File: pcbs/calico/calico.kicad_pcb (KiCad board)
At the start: 2 copper layers, 135 x 102.1 mm, 61 parts, among them J1 MJ-4PP-9-kbd-corne-light-resc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, SW1 SW_Push, SW10 SW_Push, SW11 SW_Push, SW12 SW_Push, SW13 SW_Push, SW14 SW_Push, SW15 SW_Push, SW16 SW_Push, SW17 SW_Push, SW18 SW_Push, SW19 SW_Push, SW2 SW_Push, SW20 SW_Push, SW21 SW_Push, SW22 SW_Push, SW23 SW_Push, SW24 SW_Push, SW25 SW_Push, SW26 SW_Push, SW27 SW_Push, SW3 SW_Push, SW4 SW_Push, SW5 SW_Push, SW6 SW_Push, SW7 SW_Push, SW8 SW_Push, SW9 SW_Push

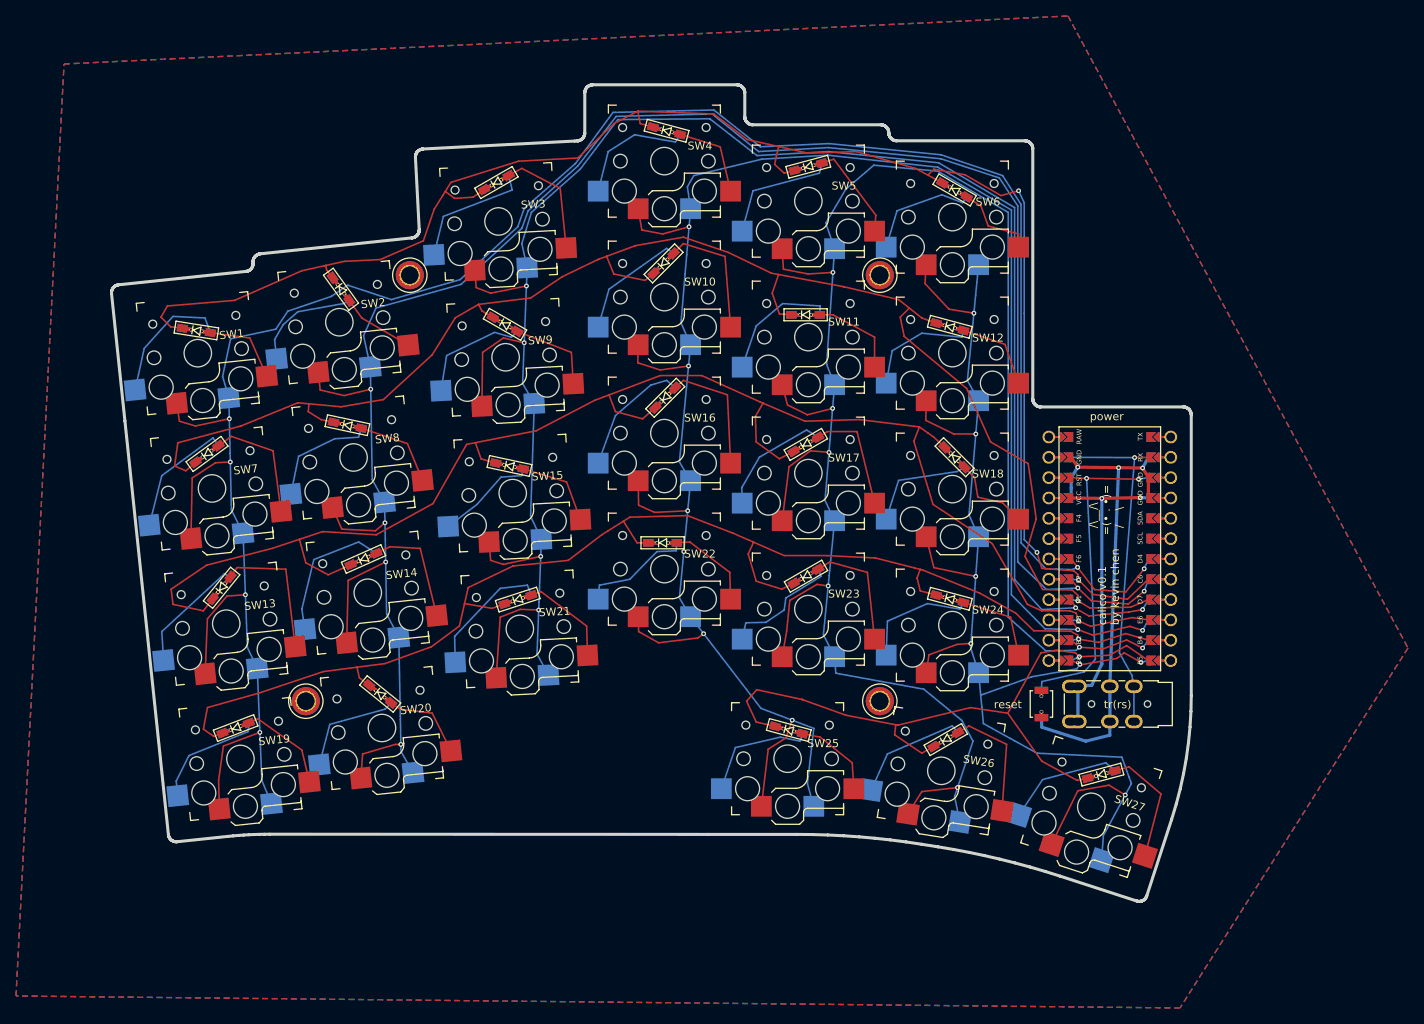
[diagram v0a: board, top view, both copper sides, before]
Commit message: v0.2 initial
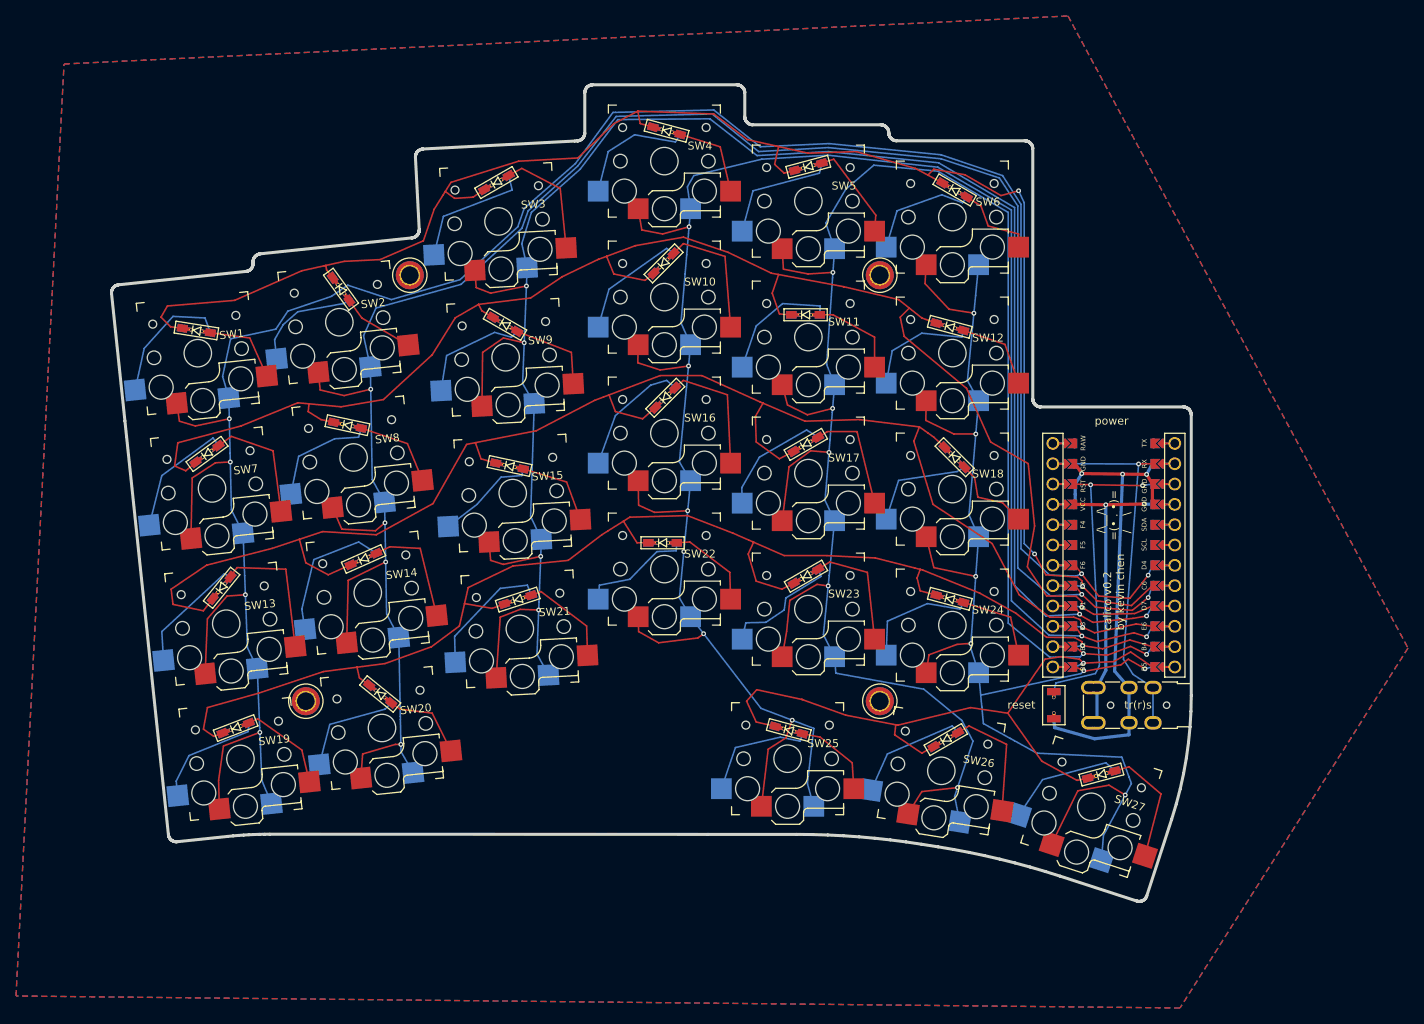
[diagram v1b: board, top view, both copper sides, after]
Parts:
- J1: footprint calico:TRRS-3pin -> calico:TRRS-3pin_modified
- RSW1: footprint calico:Reset -> calico:Reset_modified
- U1: footprint calico:ProMicro_jumpers_modified -> calico:ProMicro_jumpers
- moved J1 2.39 mm to (158.6, 95.0)
- moved RSW1 1.56 mm to (143.0, 95.0)
- moved U1 0.94 mm to (150.5, 76.2)
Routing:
- net +5V: track 39.4 -> 37.2 mm
- net /RESET: track 41.0 -> 39.6 mm
- net /COL1: track 238.3 -> 239.4 mm
- net /COL4: track 258.1 -> 259.2 mm
- net /COL2: track 248.7 -> 249.9 mm
- net /COL5: track 286.3 -> 287.4 mm
- net /COL3: track 237.6 -> 238.7 mm
- net /ROW4: track 205.4 -> 206.4 mm
- net /ROW3: track 191.4 -> 192.2 mm
- net /ROW2: track 192.0 -> 192.7 mm
- net /ROW1: track 164.0 -> 164.7 mm
- net /RX: track 43.2 -> 43.8 mm
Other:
- board text added: "calico v0.2 by kevin chen"
- board text removed: "calico v0.1 by kevin chen"
- board text removed: "tr(rs)"

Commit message: v0.2 updated
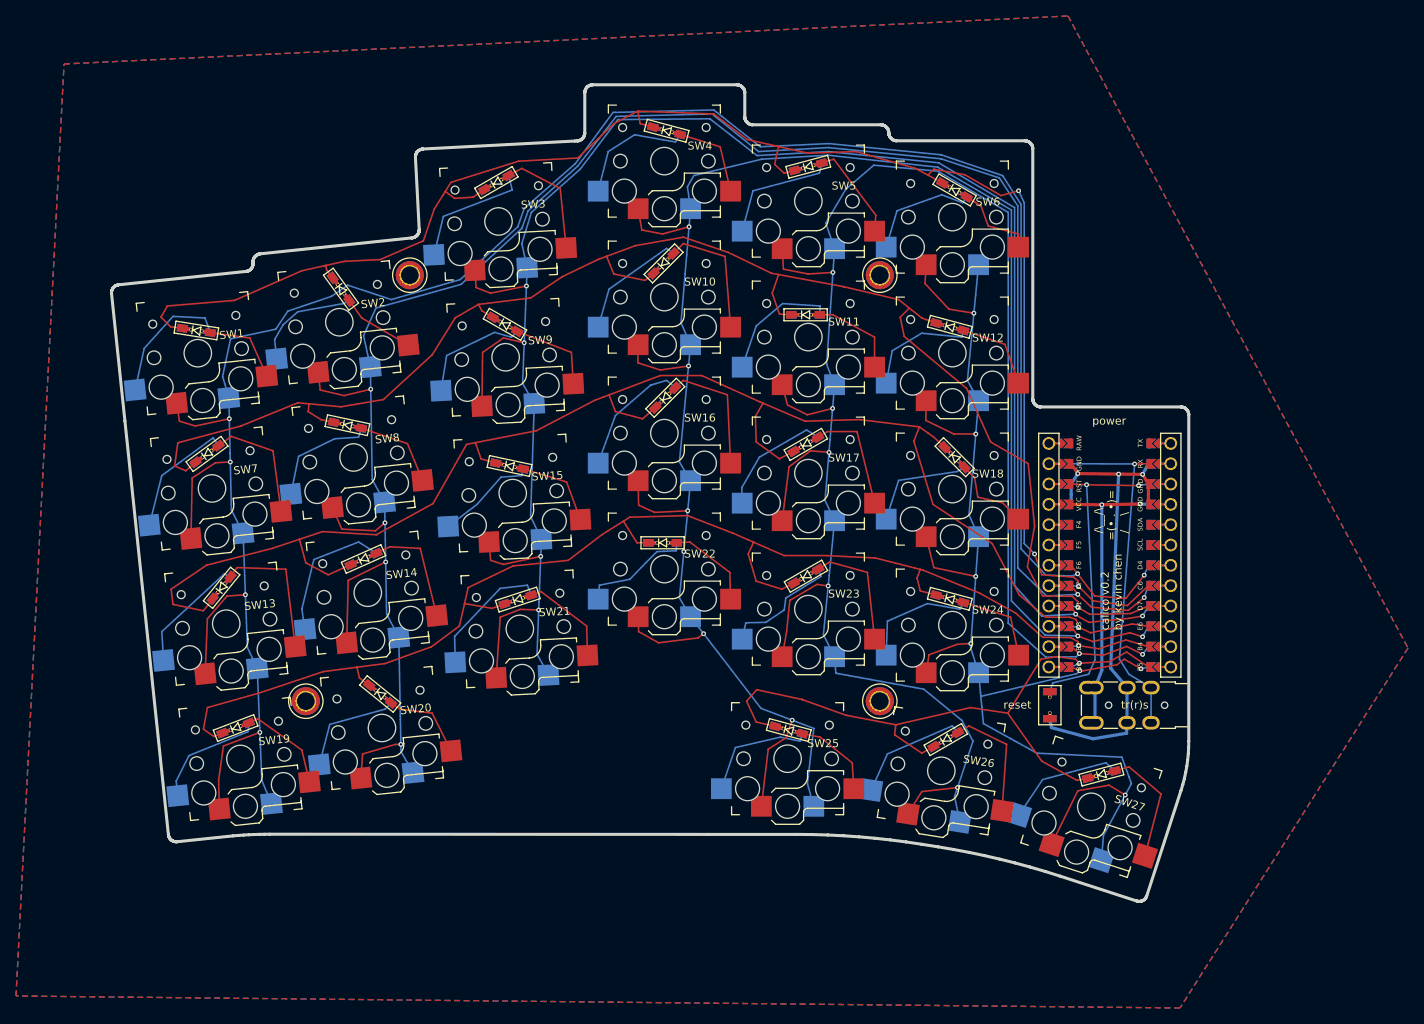
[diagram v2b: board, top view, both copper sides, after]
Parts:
- moved RSW1 0.50 mm to (142.5, 95.0)
- moved U1 0.50 mm to (150.0, 76.2)
- moved J1 0.25 mm to (158.3, 95.0)
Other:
- board size 135 x 102.1 mm -> 134.7 x 102.1 mm
